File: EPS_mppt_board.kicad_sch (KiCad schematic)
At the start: 0 parts

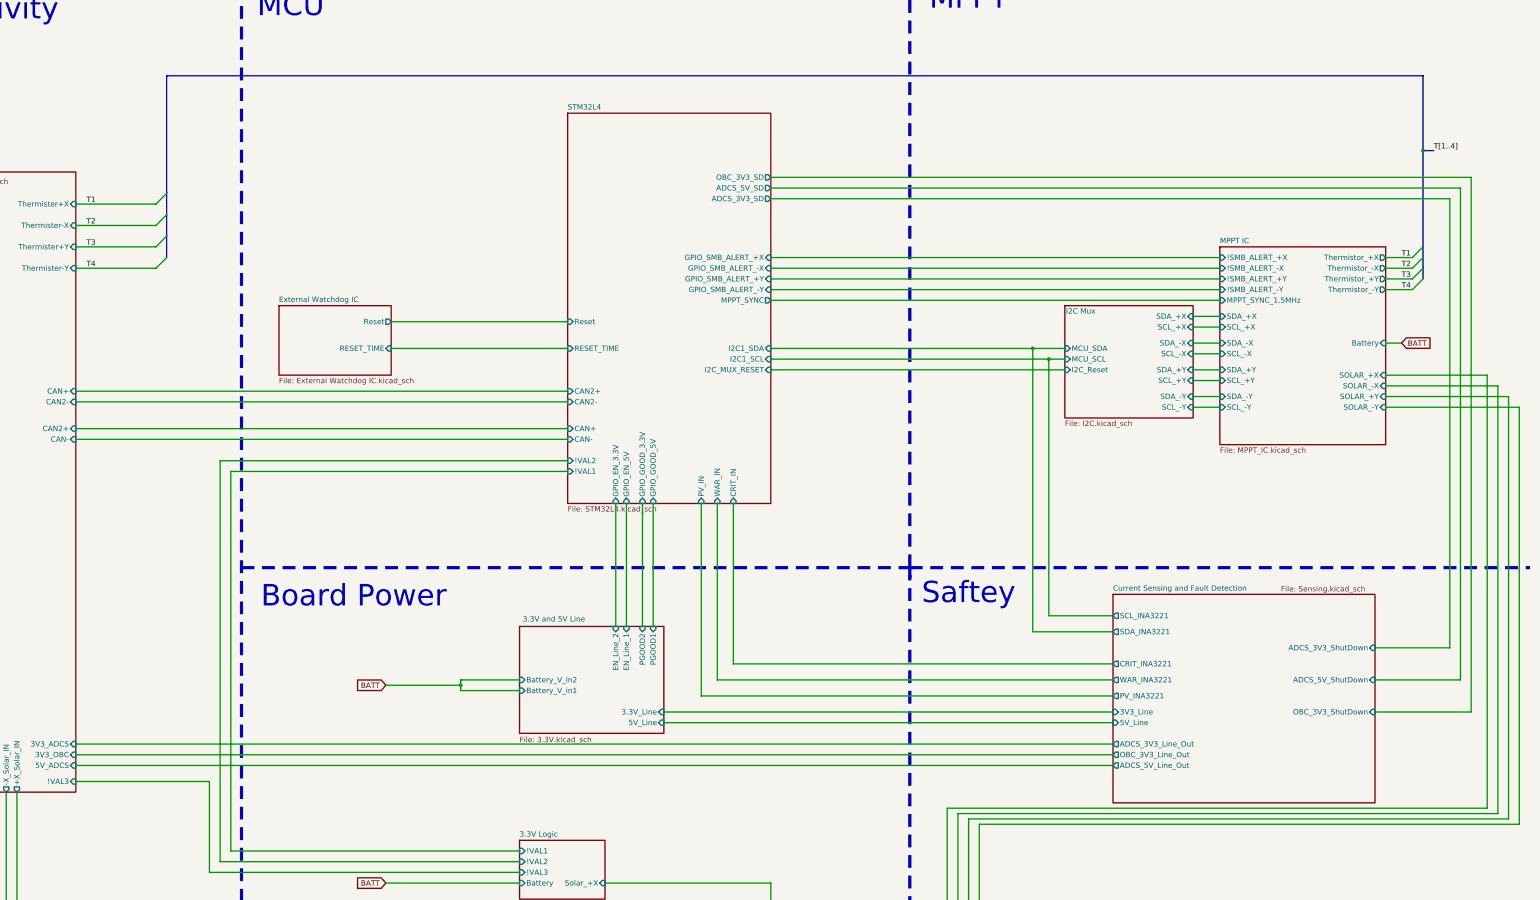
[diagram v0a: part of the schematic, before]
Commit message: Started PCB layout
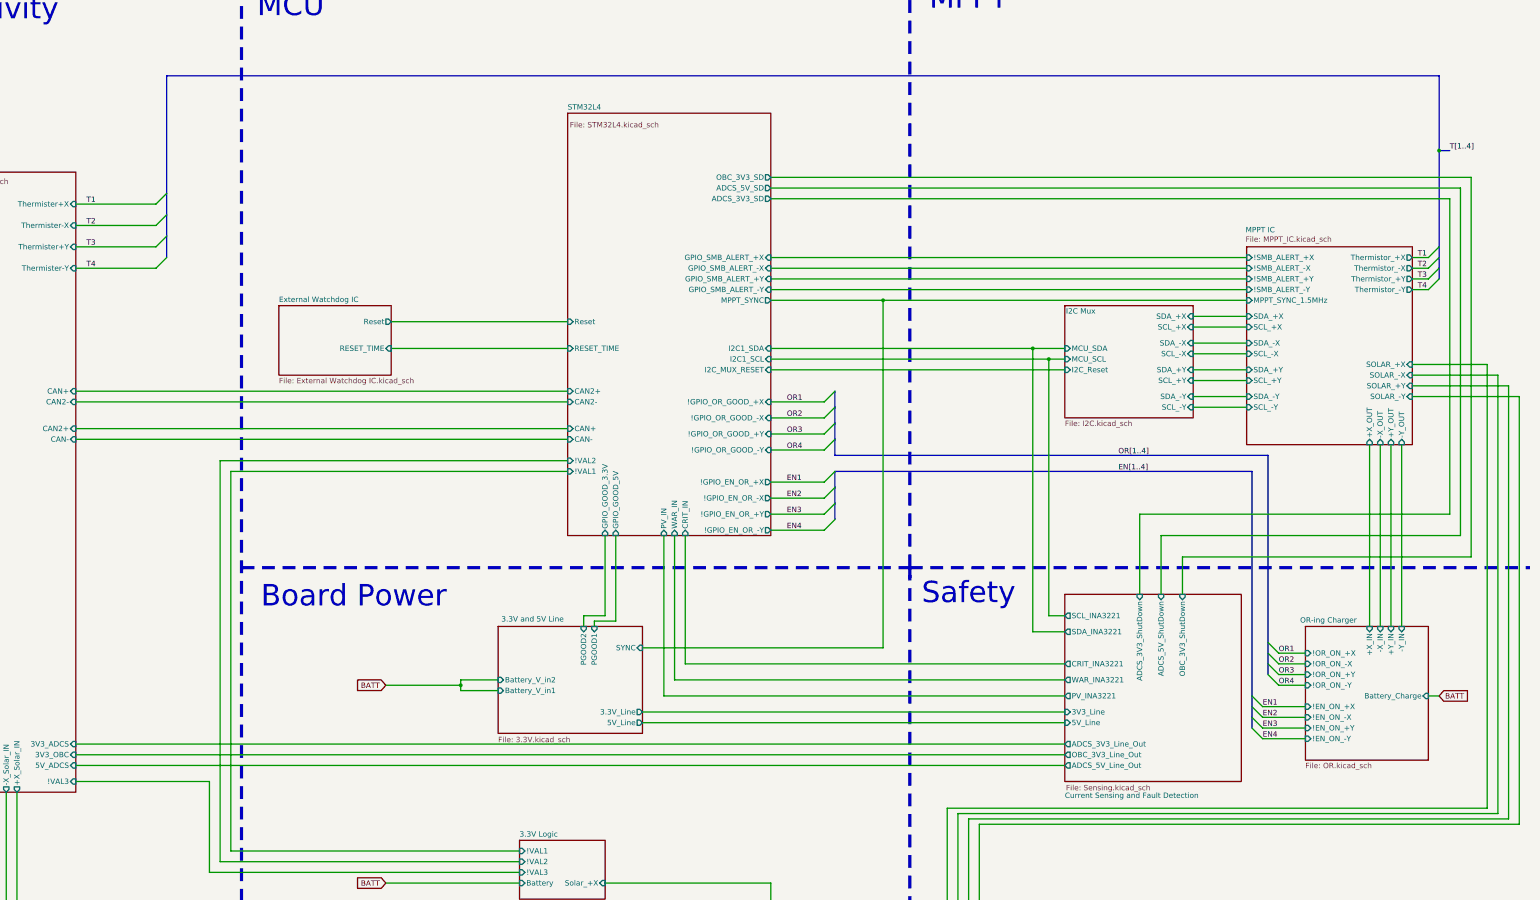
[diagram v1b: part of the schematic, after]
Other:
- added sheet OR-ing Charger (OR.kicad_sch)
- sheet 3.3V and 5V Line ports: added SYNC; removed EN_Line_1, EN_Line_2
- sheet MPPT IC ports: added +X_OUT, +Y_OUT, -X_OUT, -Y_OUT; removed Battery
- sheet STM32L4 ports: added !GPIO_EN_OR_+X, !GPIO_EN_OR_+Y, !GPIO_EN_OR_-X, !GPIO_EN_OR_-Y, !GPIO_OR_GOOD_+X, !GPIO_OR_GOOD_+Y, !GPIO_OR_GOOD_-X, !GPIO_OR_GOOD_-Y; removed GPIO_EN_3.3V, GPIO_EN_5V
- note added: "Safety"
- note removed: "Saftey"
